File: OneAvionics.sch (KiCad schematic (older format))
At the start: 43 parts, among them J1 Conn_01x02, J2 USB_B_Micro, J3 SWD, SW1 SW_SPDT, SW2 SW_SPDT, SW3 SW_Push, U1 STM32F103C8Tx, U3 LM1117-3.3, U5 LM1117-3.3, Y1 16MHz

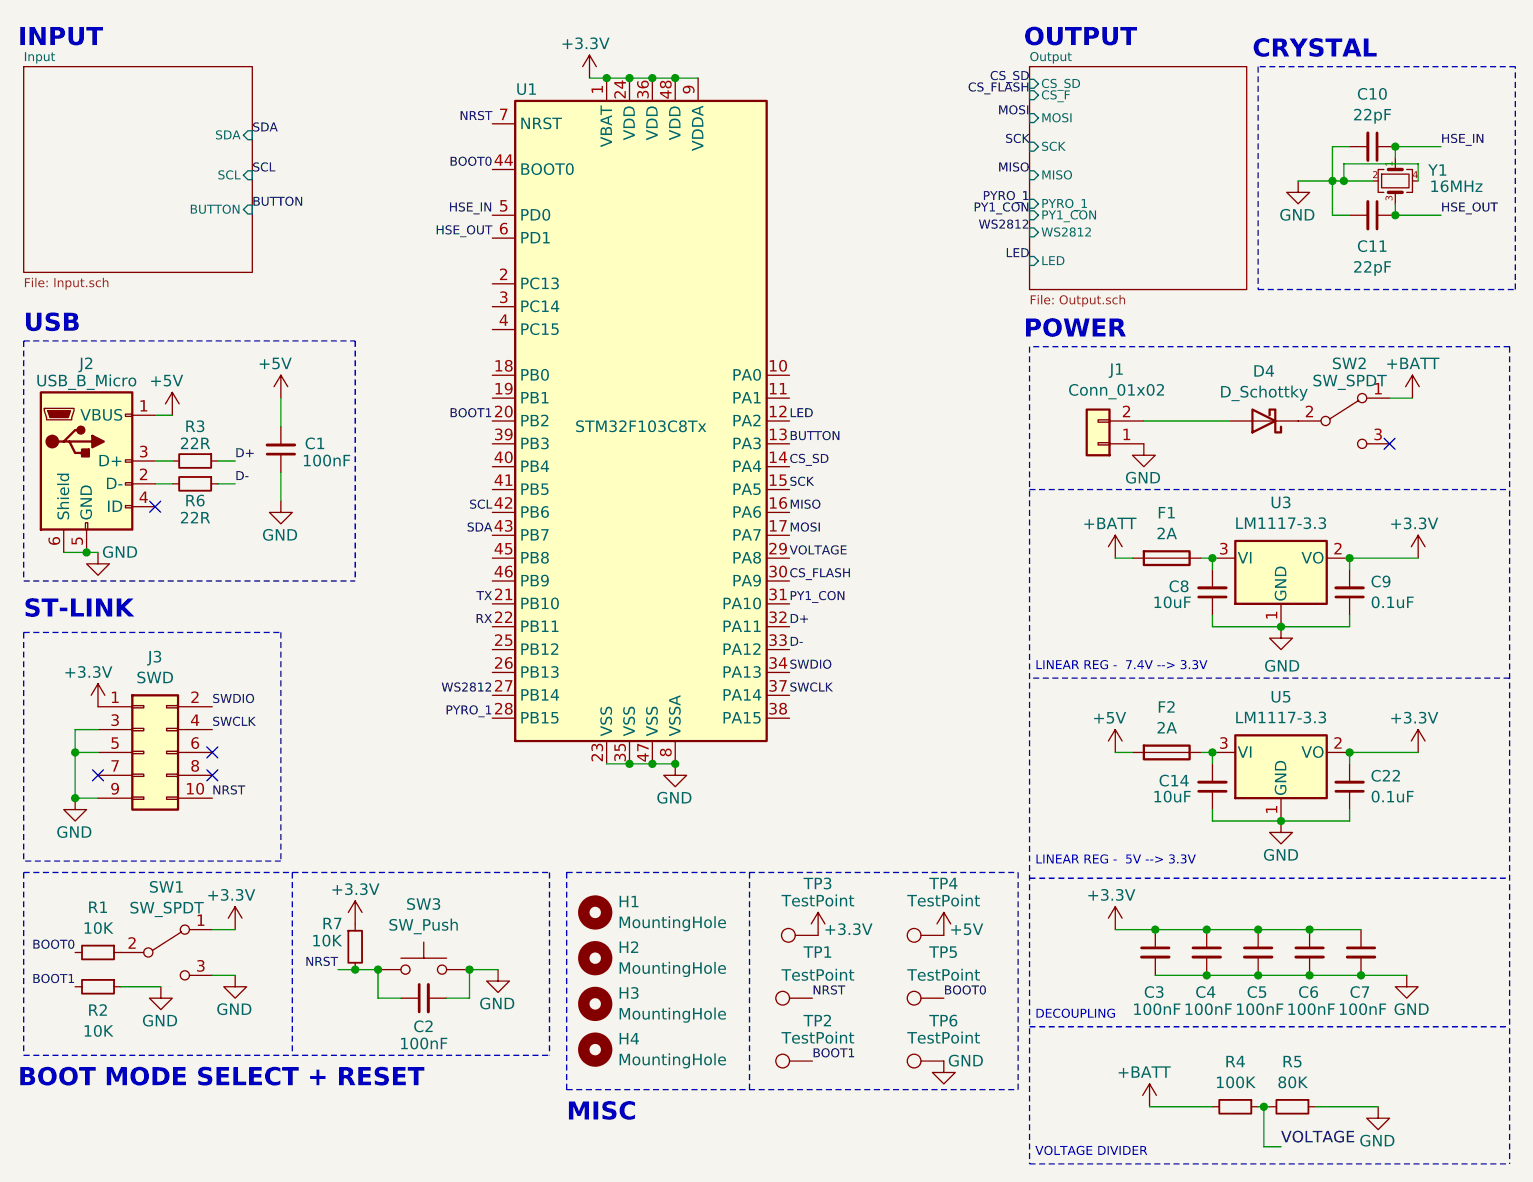
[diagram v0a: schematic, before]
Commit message: MOAR CLEANUP
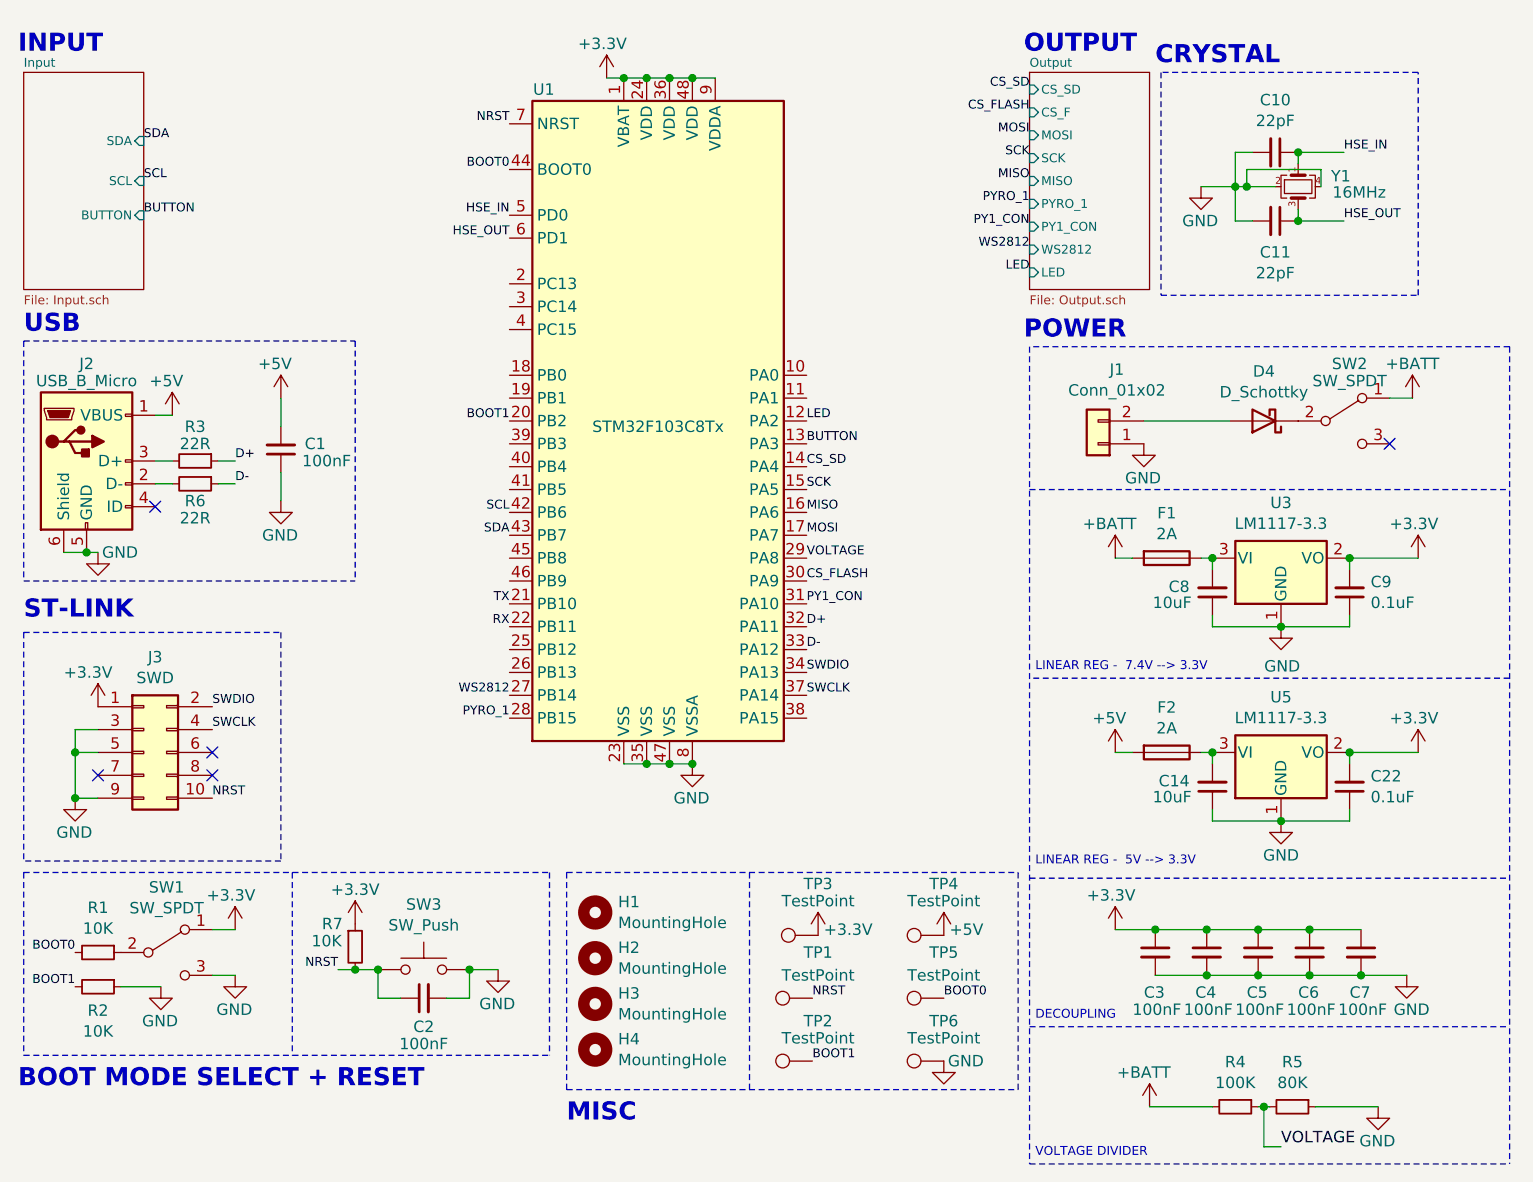
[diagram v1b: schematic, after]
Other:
- moved on the sheet: C10, C11, U1, Y1
